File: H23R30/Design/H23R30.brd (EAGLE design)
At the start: 34.6 x 30 mm, 21 parts, among them P1 HEXABIT_17.32_NO_P4_P10_P11, U1 STM32F091CBU6, X1 XTALL_CSTCE8M00G52

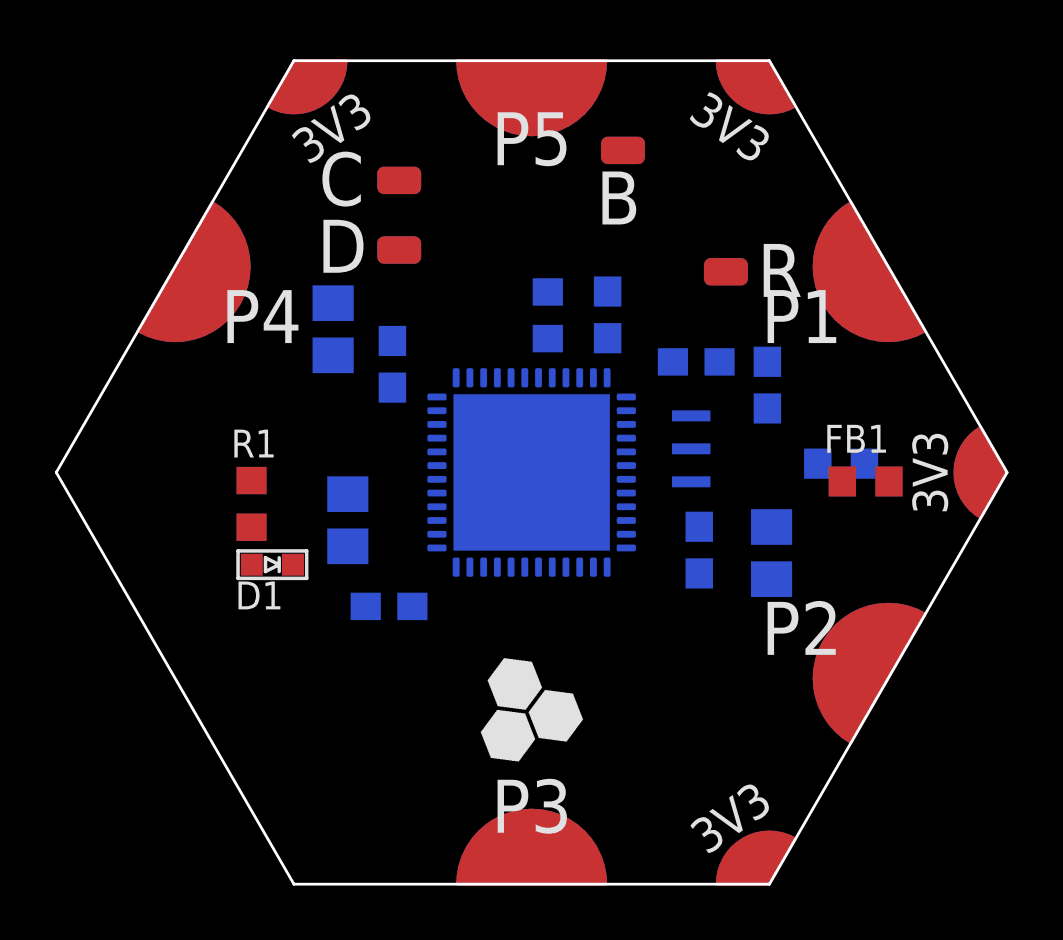
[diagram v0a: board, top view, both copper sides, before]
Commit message: Bluetooth BlueNRG module
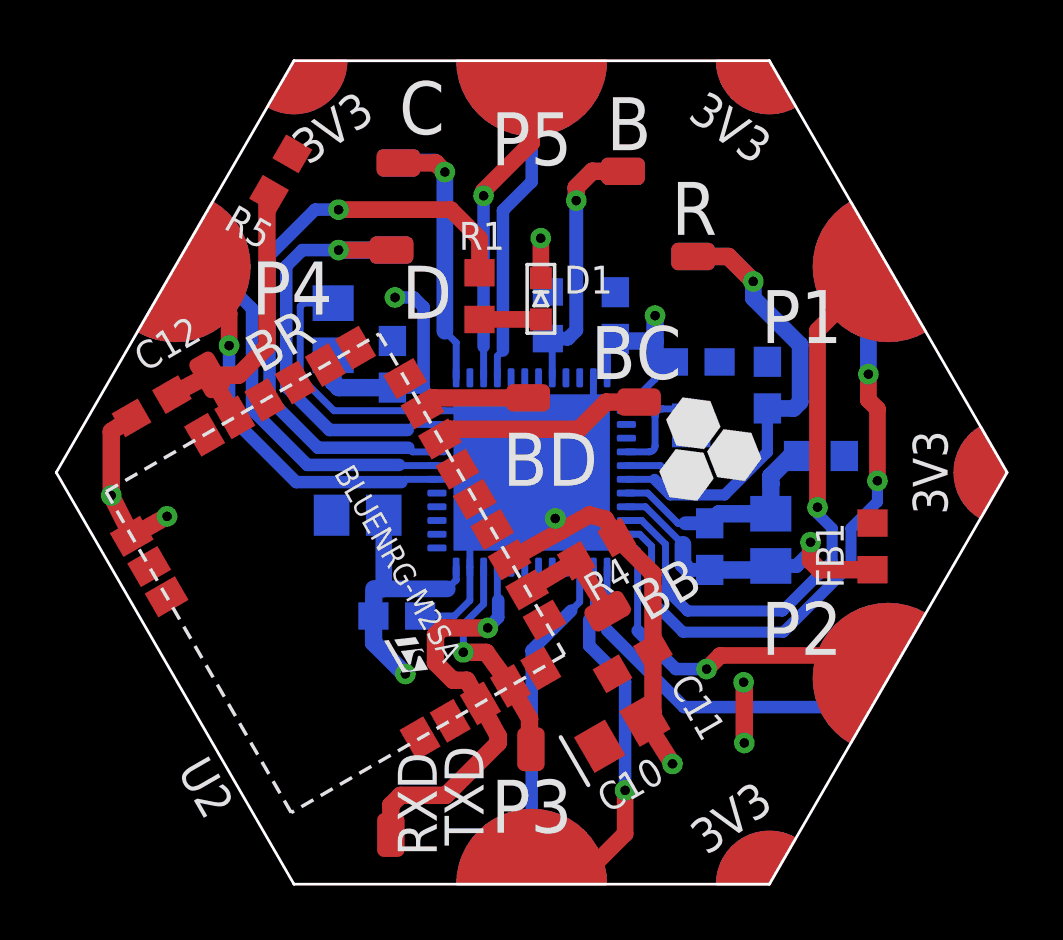
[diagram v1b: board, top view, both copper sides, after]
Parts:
- added BB, BC, BD, BR, RXD, TXD: PAD4, HEXABITZ_CONNECTION_PARTS:PAD4
- added C10: 4.7uF, HEXABITZ_RCLS:C-0805-POL
- added C11, C12: 100nF, HEXABITZ_RCLS:C-0603
- added R4: 10.0K, HEXABITZ_RCLS:R-0603
- added R5: 4.7K, HEXABITZ_RCLS:R-0603
- added U2: BLUENRG-M2SA, HEXABITZ_ICs:BLURNGR-M2SA_FOOTPRINT
- moved D1 13.8 mm to (35.0, 40.9), turned to 180 degrees
- moved R1 11.2 mm to (32.7, 41.0)
- moved FB1 2.38 mm to (47.0, 31.9), turned to 90 degrees
- moved R 1.32 mm to (40.5, 42.5)
- moved R2 0.79 mm to (45.2, 35.2)
- moved B 0.76 mm to (37.9, 45.6)
- moved C 0.64 mm to (29.8, 45.9)
- moved C2 0.48 mm to (43.3, 32.2)
- moved C6 0.45 mm to (29.7, 29.4), turned to 180 degrees
- moved C4 0.41 mm to (28.3, 33.1), turned to 0 degrees
- moved C1 0.40 mm to (41.1, 31.9)
- moved C3 0.28 mm to (37.7, 40.3)
- moved D 0.28 mm to (29.5, 42.7)
- moved X1 0.25 mm to (40.4, 35.7)
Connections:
- new net B2: BB.P$1, R4.2, U2.7
- new net N$1: BD.P$1, U2.13
- new net N$2: BC.P$1, U2.12
- new net N$8: BR.P$1, C12.2, R5.1, U2.19
- net GND: now also C10.2, C11.2, C12.1, R4.1, U2.21, U2.8
- net UART1_RX: now also P1.PAD_PD5
- net UART1_TX: now also P1.PAD_PU5
- net UART2_RX: now also P1.PAD_PD2
- net UART2_TX: now also P1.PAD_PU2
- net UART3_RX: now also TXD.P$1, U2.4
- net UART3_TX: now also RXD.P$1, U2.3
- net UART4_RX: now also P1.PAD_PD1
- net UART4_TX: now also P1.PAD_PU1
- net UART5_RX: now also P1.PAD_PD6
- net UART5_TX: now also P1.PAD_PU6
- net UART6_RX: now also P1.PAD_PD3
- net UART6_TX: now also P1.PAD_PU3
- net VDD: now also C10.1, C11.1, R5.2, U2.5
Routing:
- net GND: track 0.00 -> 54.1 mm, vias 0 -> 7
- net VDD: track 0.00 -> 28.3 mm, vias 0 -> 3
- net UART4_RX: track 0.00 -> 23.0 mm, vias 0 -> 2
- net N$3: track 0.00 -> 22.2 mm, vias 0 -> 1
- net UART4_TX: track 0.00 -> 22.0 mm, vias 0 -> 1
- net R1: track 0.00 -> 19.1 mm, vias 0 -> 1
- net N$7: track 0.00 -> 16.6 mm, vias 0 -> 1
- net UART3_TX: track 0.00 -> 15.3 mm, vias 0 -> 1
- net UART1_TX: track 0.00 -> 14.3 mm, vias 0 -> 1
- net UART6_TX: track 0.00 -> 14.2 mm, vias 0 -> 1
- net UART1_RX: track 0.00 -> 14.0 mm
- net UART2_RX: track 0.00 -> 13.7 mm
- net UART2_TX: track 0.00 -> 12.9 mm, vias 0 -> 1
- net B1: track 0.00 -> 12.2 mm, vias 0 -> 1
- net VDDA: track 0.00 -> 12.0 mm, vias 0 -> 1
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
